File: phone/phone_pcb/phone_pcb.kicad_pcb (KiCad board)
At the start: 2 copper layers, 3 parts, among them J1 Raspberry_Pi_2_3

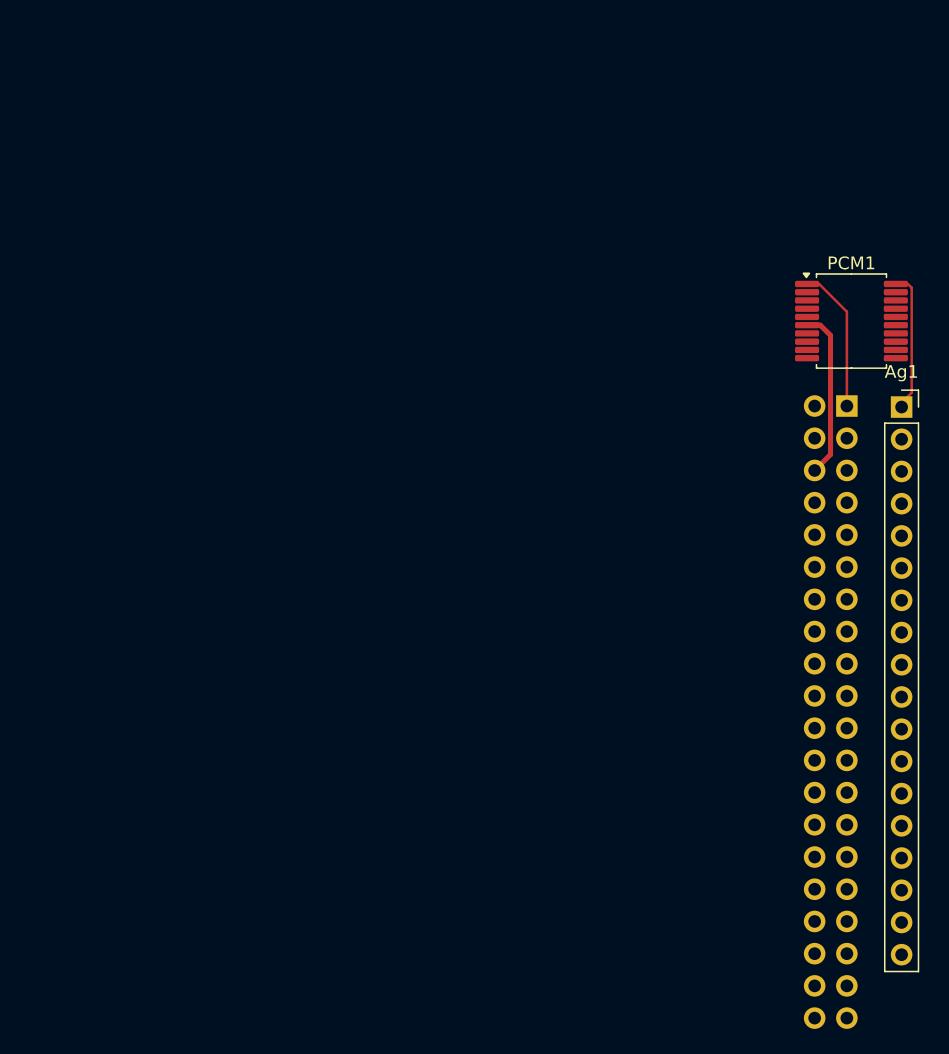
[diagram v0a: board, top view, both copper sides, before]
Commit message: Design the PCB!
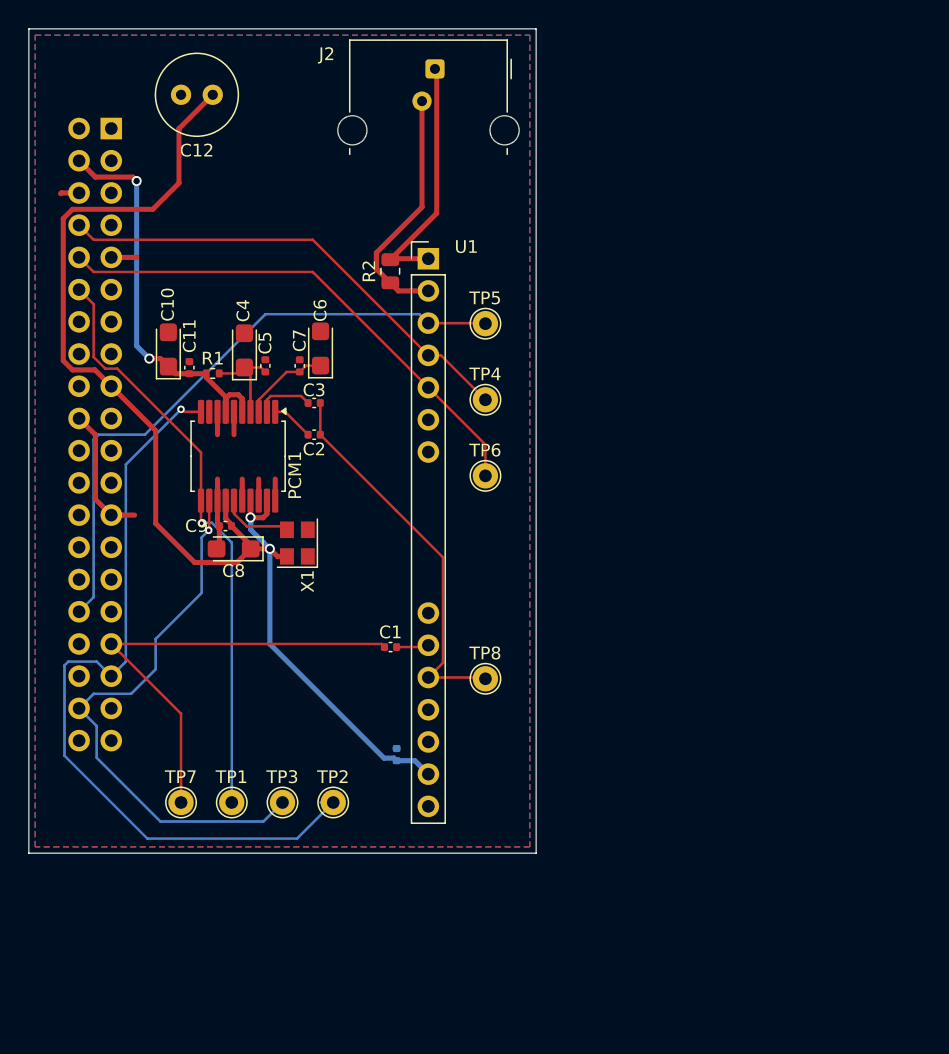
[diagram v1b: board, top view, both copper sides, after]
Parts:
- added C1: 10n, Capacitor_SMD:C_0402_1005Metric, F.Cu at (78.5, 98.7)
- added C10: 10u, Capacitor_Tantalum_SMD:CP_EIA-3216-18_Kemet-A, F.Cu at (61.0, 75.3)
- added C11: 100n, Capacitor_SMD:C_0402_1005Metric, F.Cu at (62.7, 76.7)
- added C12: 470u, Capacitor_THT:C_Radial_D6.3mm_H7.0mm_P2.50mm, F.Cu at (64.5, 55.2)
- added C13: 100n, Capacitor_SMD:C_0402_1005Metric, B.Cu at (79.0, 107.2)
- added C2: 1uF, Capacitor_SMD:C_0402_1005Metric, F.Cu at (72.5, 82.0)
- added C3: 1uF, Capacitor_SMD:C_0402_1005Metric, F.Cu at (72.5, 79.5)
- added C4: 10u, Capacitor_Tantalum_SMD:CP_EIA-3216-18_Kemet-A, F.Cu at (67.0, 75.3)
- added C5: 100n, Capacitor_SMD:C_0402_1005Metric, F.Cu at (68.6, 76.6)
- added C6: 10u, Capacitor_Tantalum_SMD:CP_EIA-3216-18_Kemet-A, F.Cu at (73.0, 75.2)
- added C7: 100n, Capacitor_SMD:C_0402_1005Metric, F.Cu at (71.4, 76.6)
- added C8: 10u, Capacitor_Tantalum_SMD:CP_EIA-3216-18_Kemet-A, F.Cu at (66.2, 91.0)
- added C9: 100n, Capacitor_SMD:C_0402_1005Metric, F.Cu at (65.5, 89.2)
- added J2: RJ11, Connector_RJ:RJ11_Ckmtw_A800_Horizontal, F.Cu at (82.0, 53.2)
- added R1: 1k, Resistor_SMD:R_0402_1005Metric, F.Cu at (64.5, 77.2)
- added R2: 20k, Resistor_SMD:R_0805_2012Metric, F.Cu at (78.5, 69.1)
- added TP1: PCM_{CLK}, TestPoint:TestPoint_THTPad_D2.0mm_Drill1.0mm, F.Cu at (66.0, 111.0)
- added TP2: PCM_{FS}, TestPoint:TestPoint_THTPad_D2.0mm_Drill1.0mm, F.Cu at (74.0, 111.0)
- added TP3: PCM_{DIN}, TestPoint:TestPoint_THTPad_D2.0mm_Drill1.0mm, F.Cu at (70.0, 111.0)
- added TP4: RM, TestPoint:TestPoint_THTPad_D2.0mm_Drill1.0mm, F.Cu at (86.0, 79.2)
- added TP5: FR, TestPoint:TestPoint_THTPad_D2.0mm_Drill1.0mm, F.Cu at (86.0, 73.2)
- added TP6: SHK, TestPoint:TestPoint_THTPad_D2.0mm_Drill1.0mm, F.Cu at (86.0, 85.2)
- added TP7: Phones, TestPoint:TestPoint_THTPad_D2.0mm_Drill1.0mm, F.Cu at (62.0, 111.0)
- added TP8: ADC_{IN}, TestPoint:TestPoint_THTPad_D2.0mm_Drill1.0mm, F.Cu at (86.0, 101.2)
- added X1: ASE-24.576MHz, Oscillator:Oscillator_SMD_Abracon_ASE-4Pin_3.2x2.5mm, F.Cu at (71.2, 90.5)
- PCM1: value ~ -> PCM1802
- U1: renamed from Ag1; value ~ -> Ag1171S; footprint Connector_PinSocket_2.54mm:PinSocket_1x18_P2.54mm_Vertical -> Connector_PinHeader_2.54mm:PinHeader_1x7+7_P2.54mm_Vertical
- moved J1 62.0 mm to (56.5, 57.9)
- moved PCM1 49.5 mm to (66.5, 83.7), turned to -90 degrees
- moved U1 39.1 mm to (81.5, 68.1)
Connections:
- J1 pad 1: Net-(PCM1-V_{IN}L) -> +3.3V
- J1 pad 10: unconnected-(J1-GPIO15/RXD-Pad10) -> /SHK
- J1 pad 12: unconnected-(J1-GPIO18/PWM0-Pad12) -> /PCM_{CLK}
- J1 pad 14: Net-(PCM1-AGND) -> GND
- J1 pad 17: Net-(PCM1-V_{IN}L) -> +3.3V
- J1 pad 2: Net-(J1-5V-Pad2) -> +5V
- J1 pad 20: Net-(PCM1-AGND) -> GND
- J1 pad 25: Net-(PCM1-AGND) -> GND
- J1 pad 30: Net-(PCM1-AGND) -> GND
- J1 pad 32: unconnected-(J1-PWM0/GPIO12-Pad32) -> /FR
- J1 pad 33: unconnected-(J1-PWM1/GPIO13-Pad33) -> Net-(J1-PWM1/GPIO13)
- J1 pad 34: Net-(PCM1-AGND) -> GND
- J1 pad 35: unconnected-(J1-GPIO19/MISO1-Pad35) -> /PCM_{FS}
- J1 pad 38: unconnected-(J1-GPIO20/MOSI1-Pad38) -> /PCM_{DIN}
- J1 pad 39: Net-(PCM1-AGND) -> GND
- J1 pad 4: Net-(J1-5V-Pad2) -> +5V
- J1 pad 6: Net-(PCM1-AGND) -> GND
- J1 pad 8: unconnected-(J1-GPIO14/TXD-Pad8) -> /RM
- J1 pad 9: Net-(PCM1-AGND) -> GND
- PCM1 pad 10: unconnected-(PCM1-LRCK-Pad10) -> /PCM_{FS}
- PCM1 pad 11: unconnected-(PCM1-BCK-Pad11) -> /PCM_{CLK}
- PCM1 pad 12: unconnected-(PCM1-D_{OUT}-Pad12) -> /PCM_{DIN}
- PCM1 pad 13: Net-(PCM1-AGND) -> GND
- PCM1 pad 14: unconnected-(PCM1-V_{DD}-Pad14) -> +3.3V
- PCM1 pad 15: unconnected-(PCM1-SCKI-Pad15) -> Net-(PCM1-SCKI)
- PCM1 pad 16: unconnected-(PCM1-OSR-Pad16) -> GND
- PCM1 pad 17: unconnected-(PCM1-FMT0-Pad17) -> +3.3V
- PCM1 pad 18: unconnected-(PCM1-FMT1-Pad18) -> GND
- PCM1 pad 19: unconnected-(PCM1-MODE0-Pad19) -> +3.3V
- PCM1 pad 2: unconnected-(PCM1-V_{IN}R-Pad2) -> Net-(PCM1-V_{IN}R)
- PCM1 pad 20: Net-(Ag1-RING) -> GND
- PCM1 pad 3: unconnected-(PCM1-V_{REF1}-Pad3) -> Net-(PCM1-V_{REF1})
- PCM1 pad 4: unconnected-(PCM1-V_{REF2}-Pad4) -> Net-(PCM1-V_{REF2})
- PCM1 pad 5: unconnected-(PCM1-V_{CC}-Pad5) -> +5V
- PCM1 pad 6: Net-(PCM1-AGND) -> GND
- PCM1 pad 7: unconnected-(PCM1-~{PDWN}-Pad7) -> +5V
- PCM1 pad 8: unconnected-(PCM1-BYPAS-Pad8) -> GND
- U1 pad 1: Net-(Ag1-RING) -> Net-(U1-RING)
- U1 pad 10: unconnected-(Ag1-V_{OUT}-Pad10) -> Net-(U1-V_{OUT})
- U1 pad 12: unconnected-(Ag1-GND-Pad12) -> GND
- U1 pad 13: unconnected-(Ag1-V_{DD}-Pad13) -> +3.3V
- U1 pad 2: unconnected-(Ag1-TIP-Pad2) -> Net-(U1-TIP)
- U1 pad 3: unconnected-(Ag1-FR-Pad3) -> /FR
- U1 pad 4: unconnected-(Ag1-RM-Pad4) -> /RM
- U1 pad 5: unconnected-(Ag1-SHK-Pad5) -> /SHK
- U1 pad 9: unconnected-(Ag1-V_{IN}-Pad9) -> Net-(U1-V_{IN})
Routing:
- net +3.3V: track 0.00 -> 94.6 mm, vias 0 -> 2
- net /PCM_{FS}: track 0.00 -> 62.5 mm, vias 0 -> 1
- net /FR: track 0.00 -> 49.6 mm
- net /PCM_{CLK}: track 0.00 -> 46.5 mm, vias 0 -> 1
- net /PCM_{DIN}: track 0.00 -> 44.2 mm, vias 0 -> 1
- net /SHK: track 0.00 -> 40.6 mm
- net /RM: track 0.00 -> 37.7 mm
- net Net-(J1-PWM1/GPIO13): track 0.00 -> 36.4 mm
- net +5V: track 0.00 -> 31.9 mm, vias 0 -> 2
- net Net-(U1-V_{OUT}): track 0.00 -> 30.7 mm
- net GND: track 0.00 -> 29.4 mm
- net Net-(U1-RING): track 0.00 -> 20.4 mm
- net Net-(U1-TIP): track 0.00 -> 19.5 mm
- net Net-(PCM1-AGND): track 13.4 -> 0.00 mm
- net Net-(Ag1-RING): track 10.7 -> 0.00 mm
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- added copper zone on B.Cu, net GND
- added copper zone on F.Cu, net GND
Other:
- board outline added: 40 x 65 mm

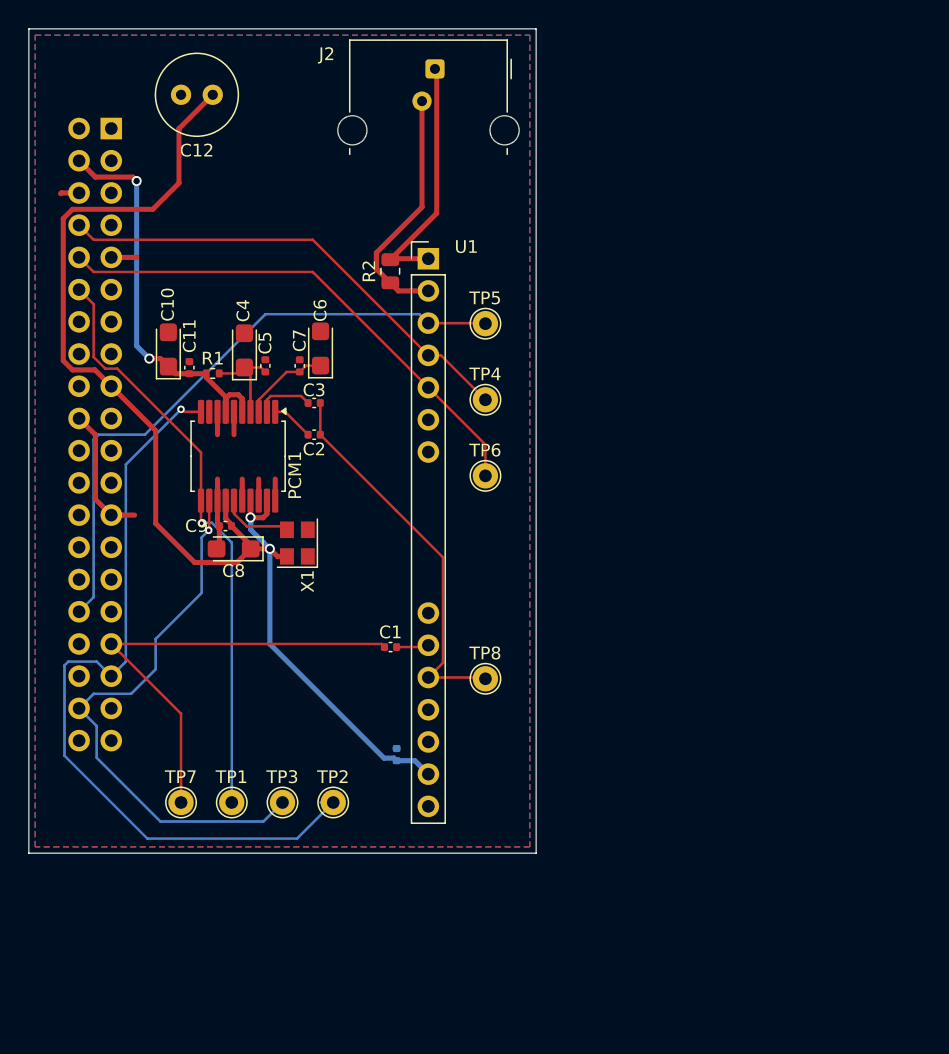
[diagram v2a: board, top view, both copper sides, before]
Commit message: Rev0.1 of PCB :D
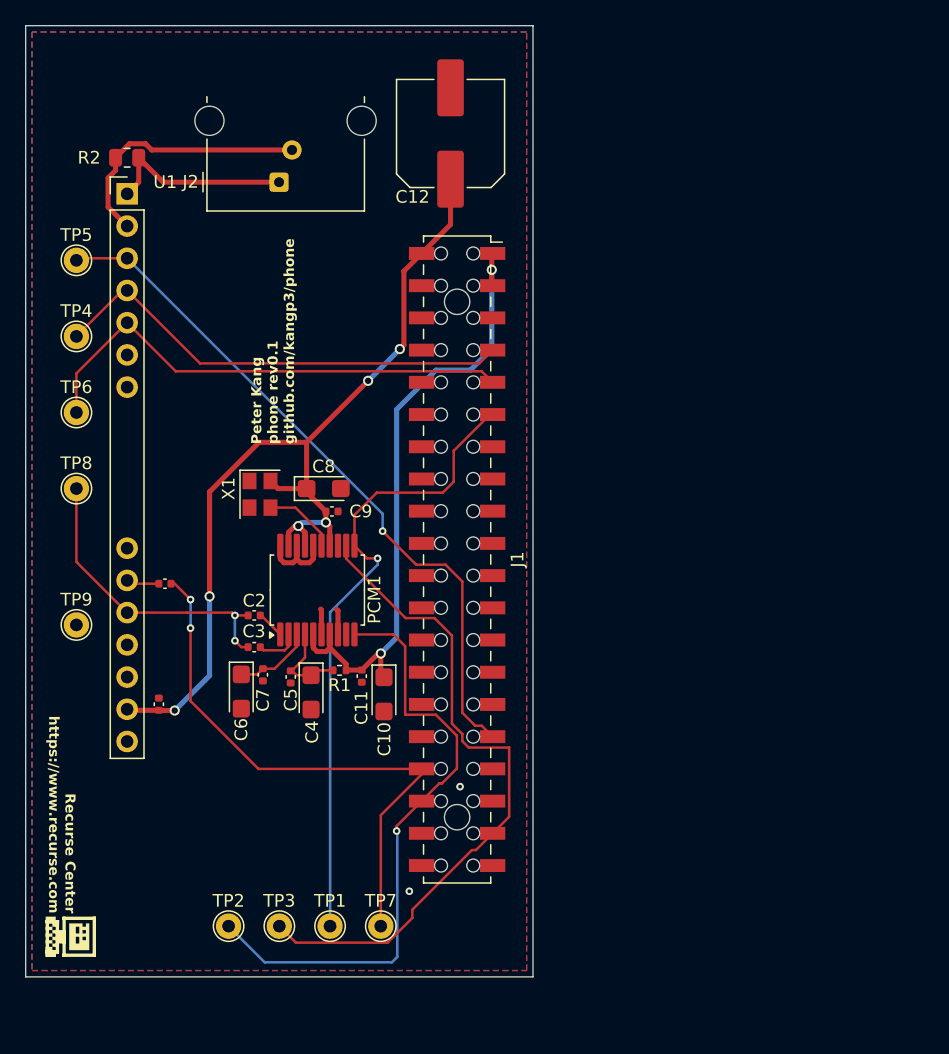
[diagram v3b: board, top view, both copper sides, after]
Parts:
- added TP9: GND, TestPoint:TestPoint_THTPad_D2.0mm_Drill1.0mm, F.Cu at (53.8, 97.0)
- C12: footprint Capacitor_THT:C_Radial_D6.3mm_H7.0mm_P2.50mm -> Capacitor_SMD:C_Elec_8x10.2
- C13: moved to F.Cu
- J1: footprint Connector_PinHeader_2.54mm:PinHeader_2x20_P2.54mm_Vertical -> Connector_Samtec_HLE_SMD:Liansheng_FH-00369_2x20_P2.54mm_Horizontal; moved to F.Cu
- moved J1 43.6 mm to (83.8, 91.8), turned to -90 degrees
- moved TP8 35.6 mm to (53.8, 86.2)
- moved TP4 32.6 mm to (53.8, 74.2)
- moved TP5 32.6 mm to (53.8, 68.2)
- moved TP6 32.6 mm to (53.8, 80.2)
- moved C10 32.1 mm to (78.0, 102.5), turned to -90 degrees
- moved C11 27.9 mm to (76.2, 101.0), turned to 90 degrees
- moved C6 27.8 mm to (66.8, 102.2), turned to -90 degrees
- moved C4 27.5 mm to (72.2, 102.3), turned to -90 degrees
- moved R1 25.5 mm to (74.5, 100.6), turned to 180 degrees
- moved C5 24.6 mm to (70.6, 101.1), turned to 90 degrees
- moved C7 24.5 mm to (68.5, 100.9), turned to 90 degrees
- moved U1 24.3 mm to (57.8, 63.0)
- moved R2 22.6 mm to (57.8, 60.2), turned to 0 degrees
- moved C3 19.8 mm to (67.8, 98.8), turned to 0 degrees
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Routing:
- net +3.3V: track 94.6 -> 75.0 mm, vias 2 -> 6
- net GND: track 29.4 -> 10.3 mm, vias 0 -> 2
- net +5V: track 31.9 -> 49.3 mm
- net /PCM_{FS}: track 62.5 -> 48.8 mm
- net /PCM_{DIN}: track 44.2 -> 53.0 mm, vias 1 -> 0
- net Net-(J1-PWM1/GPIO13): track 36.4 -> 44.2 mm, vias 0 -> 2
- net Net-(U1-V_{OUT}): track 30.7 -> 24.3 mm, vias 0 -> 2
- net /FR: track 49.6 -> 55.4 mm, vias 0 -> 1
- net Net-(U1-RING): track 20.4 -> 15.6 mm
- net /PCM_{CLK}: track 46.5 -> 50.8 mm
- net Net-(U1-TIP): track 19.5 -> 20.8 mm
- net Net-(PCM1-V_{IN}R): track 4.55 -> 3.40 mm
- net Net-(PCM1-V_{IN}L): track 3.34 -> 2.20 mm
- net /SHK: track 40.6 -> 39.5 mm
- net Net-(PCM1-V_{REF1}): track 6.94 -> 6.24 mm
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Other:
- board size 40 x 65 mm -> 40 x 75 mm
- board text added: "Peter Kang phone rev0.1 github.com/kangp3/phone"
- board text added: "Recurse Center https://www.recurse.com"

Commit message: Some PCB updates
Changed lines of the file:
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@@
 		(tags "resistor")
 		(property "Reference" "R1"
-			(at 0 -1.17 360)
+			(at 0 -1.17 0)
 			(layer "F.SilkS")
 			(effects
@@
 		)
 		(property "Value" "1k"
-			(at 0 1.17 360)
+			(at 0 1.17 0)
 			(layer "F.Fab")
 			(effects
@@
 		)
 		(fp_text user "${REFERENCE}"
-			(at 0 0 360)
+			(at 0 0 0)
 			(layer "F.Fab")
 			(effects
@@
 		(tags "capacitor")
 		(property "Reference" "C3"
-			(at -0.02 -1.25 360)
+			(at -0.02 -1.25 0)
 			(layer "F.SilkS")
 			(effects
@@
 		)
 		(property "Value" "1uF"
-			(at 0 1.16 360)
+			(at 0 1.16 0)
 			(layer "F.Fab")
 			(effects
@@
 		)
 		(fp_text user "${REFERENCE}"
-			(at 0 0 360)
+			(at 0 0 0)
 			(layer "F.Fab")
 			(effects
@@
 		(tags "resistor")
 		(property "Reference" "R2"
-			(at -3 0 360)
+			(at -3 0 0)
 			(layer "F.SilkS")
 			(effects
@@
 		)
 		(property "Value" "20k"
-			(at 0 1.65 360)
+			(at 0 1.65 0)
 			(layer "F.Fab")
 			(effects
@@
 		)
 		(fp_text user "${REFERENCE}"
-			(at 0 0 360)
+			(at 0 0 0)
 			(layer "F.Fab")
 			(effects
@@
 		(tags "capacitor")
 		(property "Reference" "C9"
-			(at -2.275 0 360)
+			(at -2.275 0 0)
 			(layer "F.SilkS")
 			(effects
@@
 		)
 		(property "Value" "100n"
-			(at 0 1.16 360)
+			(at 0 1.16 0)
 			(layer "F.Fab")
 			(hide yes)
@@
 		)
 		(fp_text user "${REFERENCE}"
-			(at 0 0 360)
+			(at 0 0 0)
 			(layer "F.Fab")
 			(effects
@@
 		(tags "capacitor tantalum")
 		(property "Reference" "C8"
-			(at 0 -1.75 360)
+			(at 0 -1.75 0)
 			(layer "F.SilkS")
 			(effects
@@
 		)
 		(property "Value" "10u"
-			(at 0 1.75 360)
+			(at 0 1.75 0)
 			(layer "F.Fab")
 			(effects
@@
 		)
 		(fp_text user "${REFERENCE}"
-			(at 0 0 360)
+			(at 0 0 0)
 			(layer "F.Fab")
 			(effects
@@
 		(tags "capacitor")
 		(property "Reference" "C2"
-			(at 0 -1.16 360)
+			(at 0 -1.16 0)
 			(layer "F.SilkS")
 			(effects
@@
 		)
 		(property "Value" "1uF"
-			(at 0 1.16 360)
+			(at 0 1.16 0)
 			(layer "F.Fab")
 			(effects
@@
 		)
 		(fp_text user "${REFERENCE}"
-			(at 0 0 360)
+			(at 0 0 0)
 			(layer "F.Fab")
 			(effects
@@
 		(tags "capacitor")
 		(property "Reference" "C1"
-			(at 0 -1.16 360)
+			(at 0 -1.16 0)
 			(layer "F.SilkS")
 			(hide yes)
@@
 		)
 		(property "Value" "10n"
-			(at 0 1.16 360)
+			(at 0 1.16 0)
 			(layer "F.Fab")
 			(hide yes)
@@
 		)
 		(fp_text user "${REFERENCE}"
-			(at 0 0 360)
+			(at 0 0 0)
 			(layer "F.Fab")
 			(effects
@@
 		(tags "RJ12 connector")
 		(property "Reference" "J2"
-			(at 7.49 -1.16 360)
+			(at 7.49 -1.16 0)
 			(layer "F.SilkS")
 			(effects
@@
 		)
 		(property "Value" "RJ11"
-			(at -0.5 12.5 360)
+			(at -0.5 12.5 0)
 			(layer "F.Fab")
 			(effects
@@
 	)
 	(gr_rect
-		(start 89.75 49.75)
-		(end 49.75 124.75)
+		(start 49.75 49.75)
+		(end 89.75 124.75)
 		(stroke
 			(width 0.05)
@@
 	)
 	(gr_rect
-		(start 89.25 50.25)
-		(end 50.25 124.25)
+		(start 50.25 50.25)
+		(end 89.25 124.25)
 		(stroke
 			(width 0.1)
